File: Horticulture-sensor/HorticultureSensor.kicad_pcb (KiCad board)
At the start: 2 copper layers, 46.9 x 34.8 mm, 15 parts, among them J1 Conn_01x04, J2 Conn_02x05_Odd_Even, J3 Conn_01x03, J4 Conn_01x04, J5 Conn_01x03, J6 Conn_01x04, U1 STM32F030F4Px

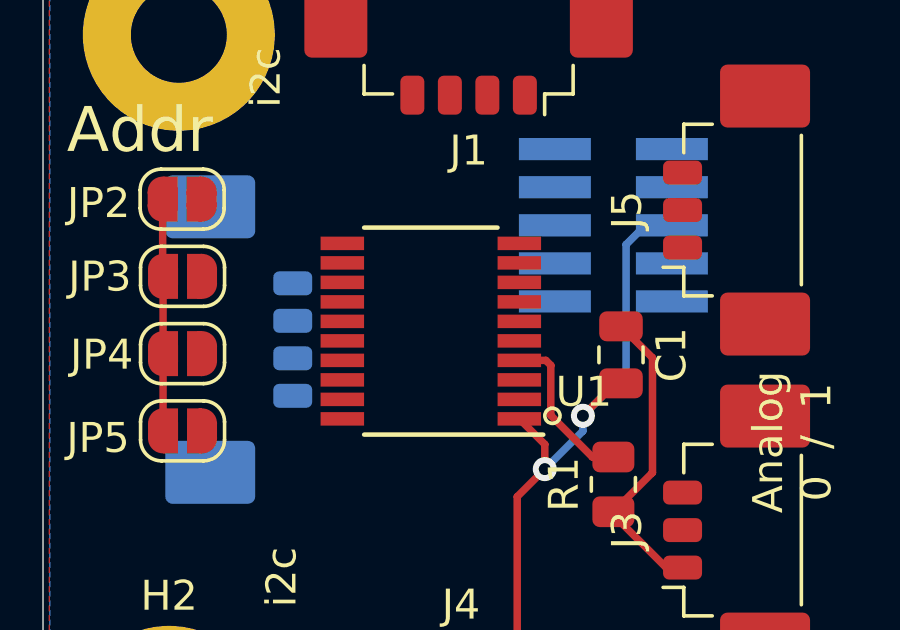
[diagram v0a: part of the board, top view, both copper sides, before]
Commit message: Resolves #2
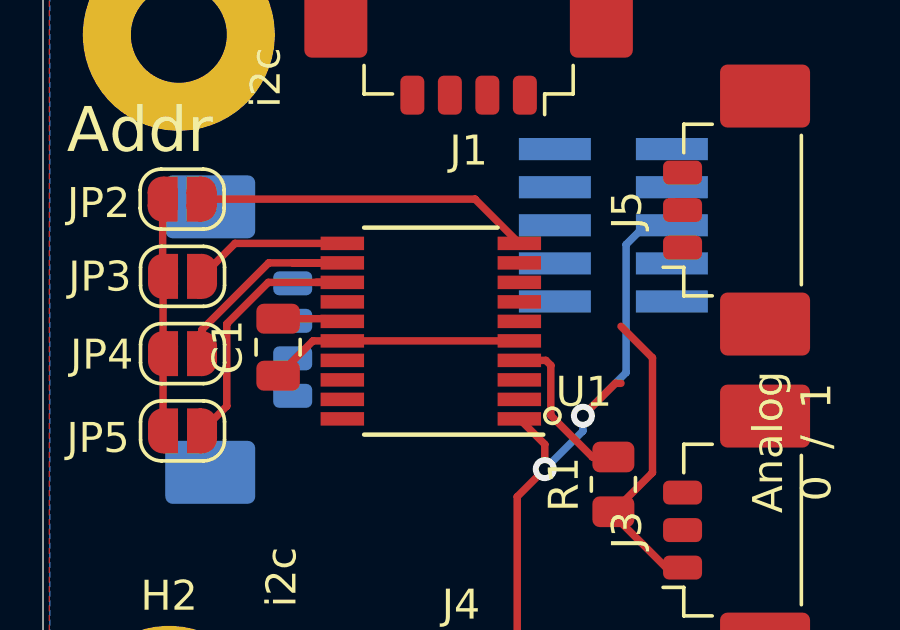
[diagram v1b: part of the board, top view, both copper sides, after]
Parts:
- moved C1 11.4 mm to (151.4, 129.3), turned to 90 degrees
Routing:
- net i2c-addr_0: track 0.00 -> 11.2 mm
- net i2c-addr_3: track 0.00 -> 9.22 mm
- net +3V3: track 10.3 -> 18.8 mm
- net i2c-addr_2: track 0.00 -> 8.09 mm
- net i2c-addr_1: track 0.00 -> 5.13 mm
- net GND: track 29.9 -> 32.6 mm
